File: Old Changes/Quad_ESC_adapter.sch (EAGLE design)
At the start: 13 parts, among them J1 IBPD-SOCKET, J2 IBPD-SOCKET, J3 IBPD-SOCKET, J4 IBPD-SOCKET

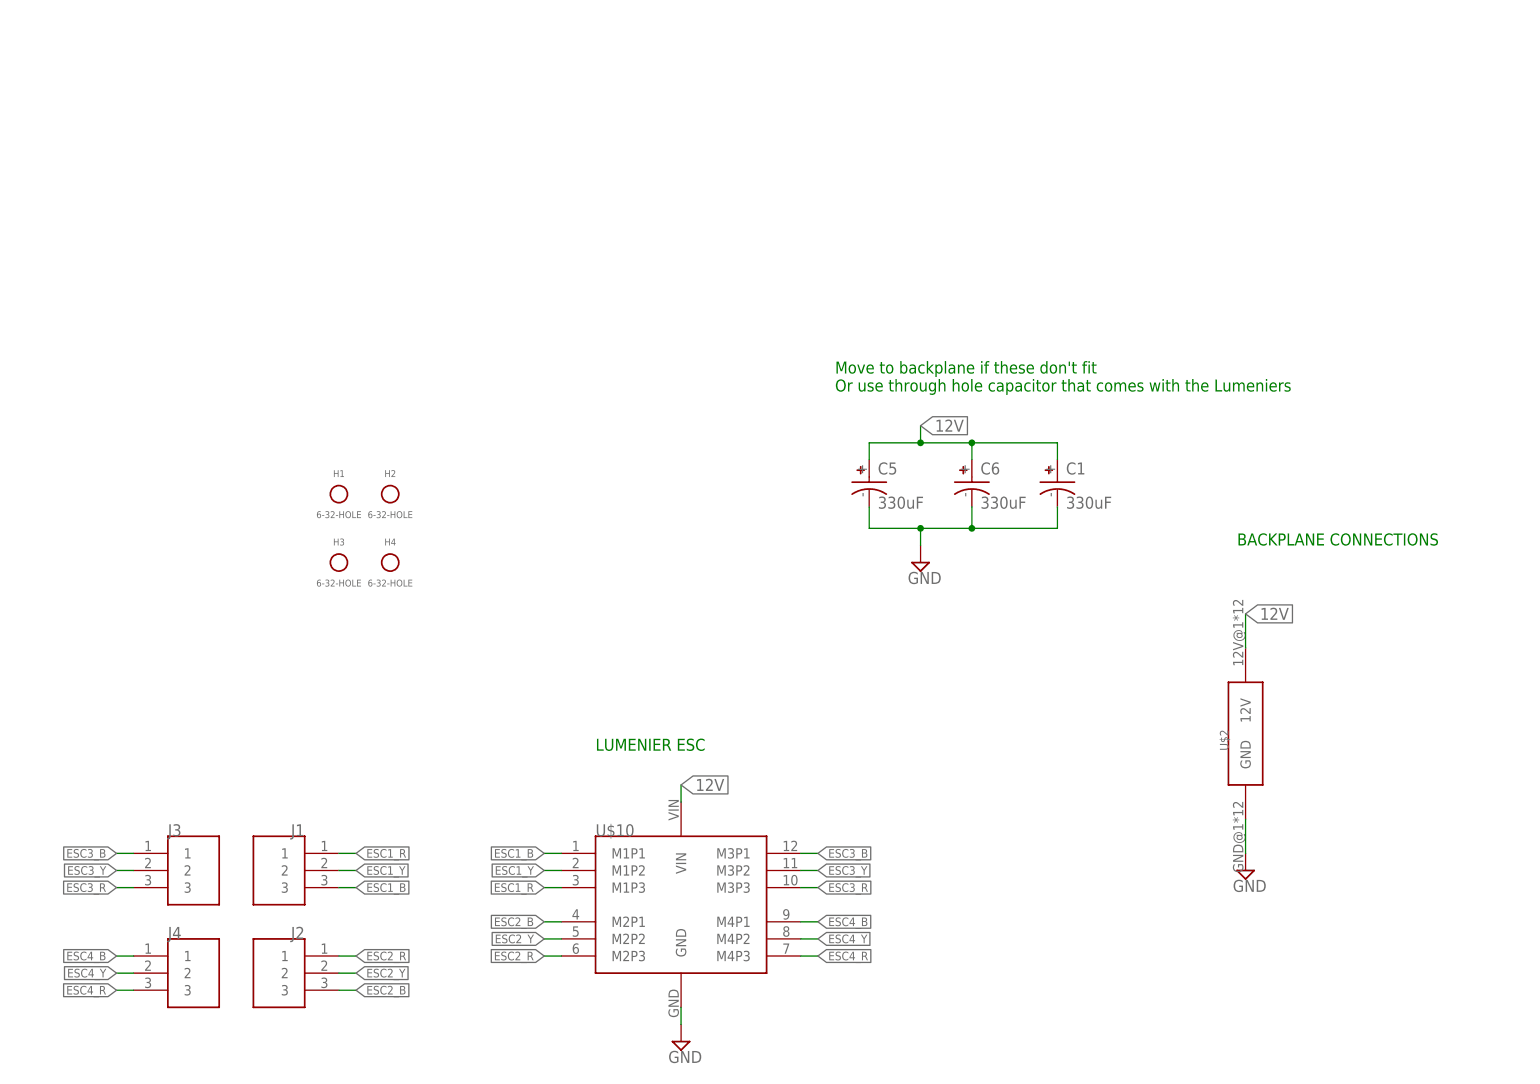
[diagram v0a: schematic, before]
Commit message: .
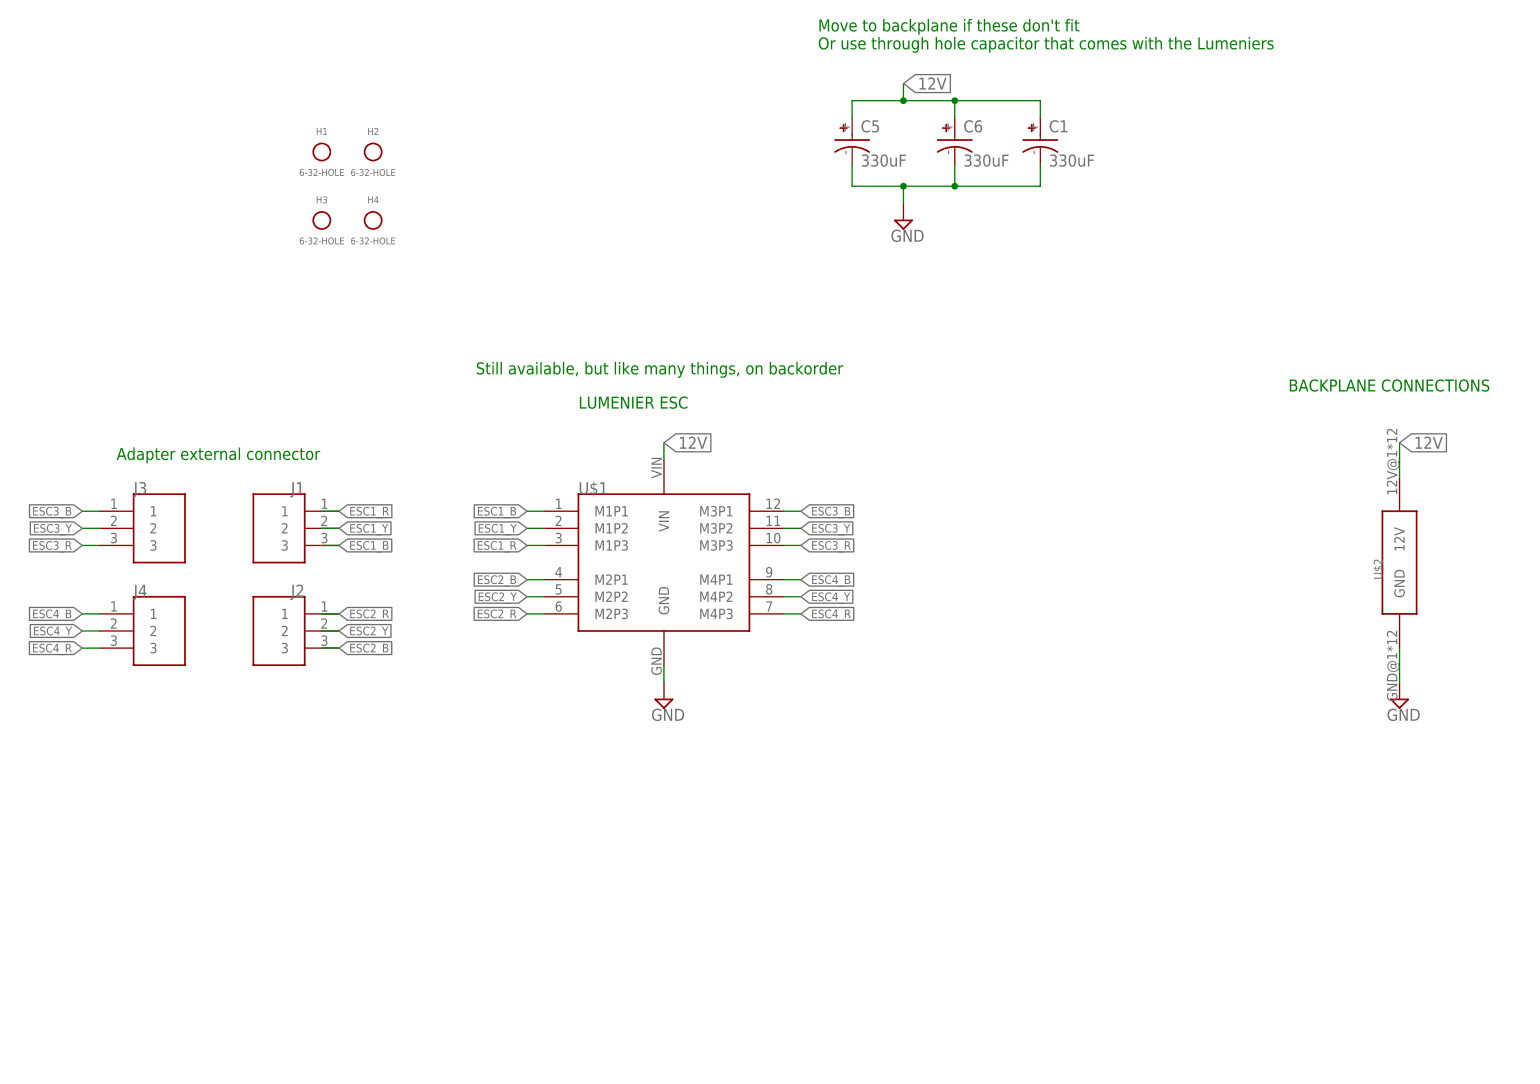
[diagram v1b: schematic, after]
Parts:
- removed U$10: LUMENIER_QUAD-NO-CUT, Lumenier ESC:LUMENIER_QUAD-NO-CUT
- added U$1: LUMENIER_QUAD, AUX, Lumenier ESC:LUMENIER_QUAD
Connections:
- net 12V: now also U$1.VIN; no longer U$10.VIN
- net ESC1_B: now also U$1.M1P1; no longer U$10.M1P1
- net ESC1_R: now also U$1.M1P3; no longer U$10.M1P3
- net ESC1_Y: now also U$1.M1P2; no longer U$10.M1P2
- net ESC2_B: now also U$1.M2P1; no longer U$10.M2P1
- net ESC2_R: now also U$1.M2P3; no longer U$10.M2P3
- net ESC2_Y: now also U$1.M2P2; no longer U$10.M2P2
- net ESC3_B: now also U$1.M3P1; no longer U$10.M3P1
- net ESC3_R: now also U$1.M3P3; no longer U$10.M3P3
- net ESC3_Y: now also U$1.M3P2; no longer U$10.M3P2
- net ESC4_B: now also U$1.M4P1; no longer U$10.M4P1
- net ESC4_R: now also U$1.M4P3; no longer U$10.M4P3
- net ESC4_Y: now also U$1.M4P2; no longer U$10.M4P2
- net GND: now also U$1.GND; no longer U$10.GND
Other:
- note added: "Adapter external connector"
- note added: "Still available, but like many things, on backorder"
- moved on the sheet: C1, C5, C6, H1, H2, H3, H4, J1, J2, J3, J4, U$2
